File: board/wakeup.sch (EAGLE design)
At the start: 41 parts, among them IC2 ATMEGA48/88/168-AU, K1 PIN20X2, Q5 BC846BSMD, Q6 BC846BSMD, Q7 BC846BSMD, Q8 BC846BSMD, U1 EEPROM24

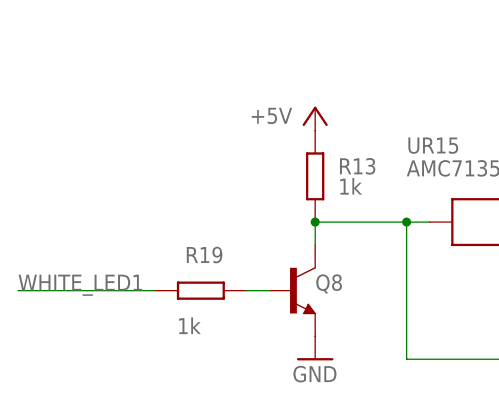
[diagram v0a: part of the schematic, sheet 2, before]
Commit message: Fixed some errors
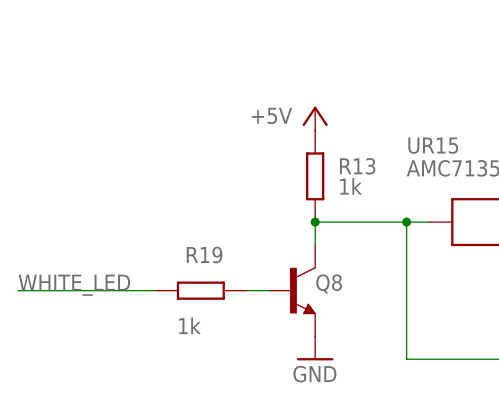
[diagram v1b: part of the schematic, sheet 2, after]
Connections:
- removed net WHITE_LED1: R19.2
- net WHITE_LED: now also R19.2
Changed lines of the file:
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@@
 <grid distance="0.1" unitdist="inch" unit="inch" style="lines" multiple="1" display="no" altdistance="0.01" altunitdist="inch" altunit="inch"/>
 <layers>
-<layer number="1" name="Top" color="4" fill="1" visible="yes" active="no"/>
-<layer number="2" name="Route2" color="1" fill="3" visible="yes" active="no"/>
-<layer number="3" name="Route3" color="4" fill="3" visible="yes" active="no"/>
-<layer number="4" name="Route4" color="1" fill="4" visible="yes" active="no"/>
-<layer number="5" name="Route5" color="4" fill="4" visible="yes" active="no"/>
-<layer number="6" name="Route6" color="1" fill="8" visible="yes" active="no"/>
-<layer number="7" name="Route7" color="4" fill="8" visible="yes" active="no"/>
-<layer number="8" name="Route8" color="1" fill="2" visible="yes" active="no"/>
-<layer number="9" name="Route9" color="4" fill="2" visible="yes" active="no"/>
-<layer number="10" name="Route10" color="1" fill="7" visible="yes" active="no"/>
-<layer number="11" name="Route11" color="4" fill="7" visible="yes" active="no"/>
-<layer number="12" name="Route12" color="1" fill="5" visible="yes" active="no"/>
-<layer number="13" name="Route13" color="4" fill="5" visible="yes" active="no"/>
-<layer number="14" name="Route14" color="1" fill="6" visible="yes" active="no"/>
-<layer number="15" name="Route15" color="4" fill="6" visible="yes" active="no"/>
-<layer number="16" name="Bottom" color="1" fill="1" visible="yes" active="no"/>
-<layer number="17" name="Pads" color="2" fill="1" visible="yes" active="no"/>
-<layer number="18" name="Vias" color="2" fill="1" visible="yes" active="no"/>
-<layer number="19" name="Unrouted" color="6" fill="1" visible="yes" active="no"/>
-<layer number="20" name="Dimension" color="15" fill="1" visible="yes" active="no"/>
-<layer number="21" name="tPlace" color="7" fill="1" visible="yes" active="no"/>
-<layer number="22" name="bPlace" color="7" fill="1" visible="yes" active="no"/>
-<layer number="23" name="tOrigins" color="15" fill="1" visible="yes" active="no"/>
-<layer number="24" name="bOrigins" color="15" fill="1" visible="yes" active="no"/>
-<layer number="25" name="tNames" color="7" fill="1" visible="yes" active="no"/>
-<layer number="26" name="bNames" color="7" fill="1" visible="yes" active="no"/>
-<layer number="27" name="tValues" color="7" fill="1" visible="yes" active="no"/>
-<layer number="28" name="bValues" color="7" fill="1" visible="yes" active="no"/>
+<layer number="1" name="Top" color="4" fill="1" visible="no" active="no"/>
+<layer number="2" name="Route2" color="1" fill="3" visible="no" active="no"/>
+<layer number="3" name="Route3" color="4" fill="3" visible="no" active="no"/>
+<layer number="4" name="Route4" color="1" fill="4" visible="no" active="no"/>
+<layer number="5" name="Route5" color="4" fill="4" visible="no" active="no"/>
+<layer number="6" name="Route6" color="1" fill="8" visible="no" active="no"/>
+<layer number="7" name="Route7" color="4" fill="8" visible="no" active="no"/>
+<layer number="8" name="Route8" color="1" fill="2" visible="no" active="no"/>
+<layer number="9" name="Route9" color="4" fill="2" visible="no" active="no"/>
+<layer number="10" name="Route10" color="1" fill="7" visible="no" active="no"/>
+<layer number="11" name="Route11" color="4" fill="7" visible="no" active="no"/>
+<layer number="12" name="Route12" color="1" fill="5" visible="no" active="no"/>
+<layer number="13" name="Route13" color="4" fill="5" visible="no" active="no"/>
+<layer number="14" name="Route14" color="1" fill="6" visible="no" active="no"/>
+<layer number="15" name="Route15" color="4" fill="6" visible="no" active="no"/>
+<layer number="16" name="Bottom" color="1" fill="1" visible="no" active="no"/>
+<layer number="17" name="Pads" color="2" fill="1" visible="no" active="no"/>
+<layer number="18" name="Vias" color="2" fill="1" visible="no" active="no"/>
+<layer number="19" name="Unrouted" color="6" fill="1" visible="no" active="no"/>
+<layer number="20" name="Dimension" color="15" fill="1" visible="no" active="no"/>
+<layer number="21" name="tPlace" color="7" fill="1" visible="no" active="no"/>
+<layer number="22" name="bPlace" color="7" fill="1" visible="no" active="no"/>
+<layer number="23" name="tOrigins" color="15" fill="1" visible="no" active="no"/>
+<layer number="24" name="bOrigins" color="15" fill="1" visible="no" active="no"/>
+<layer number="25" name="tNames" color="7" fill="1" visible="no" active="no"/>
+<layer number="26" name="bNames" color="7" fill="1" visible="no" active="no"/>
+<layer number="27" name="tValues" color="7" fill="1" visible="no" active="no"/>
+<layer number="28" name="bValues" color="7" fill="1" visible="no" active="no"/>
 <layer number="29" name="tStop" color="7" fill="3" visible="no" active="no"/>
 <layer number="30" name="bStop" color="7" fill="6" visible="no" active="no"/>
@@
 <layer number="35" name="tGlue" color="7" fill="4" visible="no" active="no"/>
 <layer number="36" name="bGlue" color="7" fill="5" visible="no" active="no"/>
-<layer number="37" name="tTest" color="7" fill="1" visible="yes" active="no"/>
-<layer number="38" name="bTest" color="7" fill="1" visible="yes" active="no"/>
+<layer number="37" name="tTest" color="7" fill="1" visible="no" active="no"/>
+<layer number="38" name="bTest" color="7" fill="1" visible="no" active="no"/>
 <layer number="39" name="tKeepout" color="4" fill="11" visible="no" active="no"/>
 <layer number="40" name="bKeepout" color="1" fill="11" visible="no" active="no"/>
@@
 <layer number="44" name="Drills" color="7" fill="1" visible="no" active="no"/>
 <layer number="45" name="Holes" color="7" fill="1" visible="no" active="no"/>
-<layer number="46" name="Milling" color="3" fill="1" visible="yes" active="no"/>
-<layer number="47" name="Measures" color="7" fill="1" visible="yes" active="no"/>
-<layer number="48" name="Document" color="7" fill="1" visible="yes" active="no"/>
-<layer number="49" name="Reference" color="7" fill="1" visible="yes" active="no"/>
-<layer number="50" name="dxf" color="7" fill="1" visible="yes" active="no"/>
-<layer number="51" name="tDocu" color="7" fill="1" visible="yes" active="no"/>
-<layer number="52" name="bDocu" color="7" fill="1" visible="yes" active="no"/>
-<layer number="53" name="tGND_GNDA" color="7" fill="1" visible="yes" active="no"/>
-<layer number="54" name="bGND_GNDA" color="7" fill="1" visible="yes" active="no"/>
-<layer number="56" name="wert" color="7" fill="1" visible="yes" active="no"/>
+<layer number="46" name="Milling" color="3" fill="1" visible="no" active="no"/>
+<layer number="47" name="Measures" color="7" fill="1" visible="no" active="no"/>
+<layer number="48" name="Document" color="7" fill="1" visible="no" active="no"/>
+<layer number="49" name="Reference" color="7" fill="1" visible="no" active="no"/>
+<layer number="50" name="dxf" color="7" fill="1" visible="no" active="no"/>
+<layer number="51" name="tDocu" color="7" fill="1" visible="no" active="no"/>
+<layer number="52" name="bDocu" color="7" fill="1" visible="no" active="no"/>
+<layer number="53" name="tGND_GNDA" color="7" fill="1" visible="no" active="no"/>
+<layer number="54" name="bGND_GNDA" color="7" fill="1" visible="no" active="no"/>
+<layer number="56" name="wert" color="7" fill="1" visible="no" active="no"/>
 <layer number="90" name="Modules" color="5" fill="1" visible="yes" active="yes"/>
 <layer number="91" name="Nets" color="2" fill="1" visible="yes" active="yes"/>
@@
 </segment>
 </net>
-<net name="WHITE_LED1" class="0">
+<net name="WHITE_LED" class="0">
 <segment>
 <wire x1="27.94" y1="38.1" x2="43.18" y2="38.1" width="0.1524" layer="91"/>

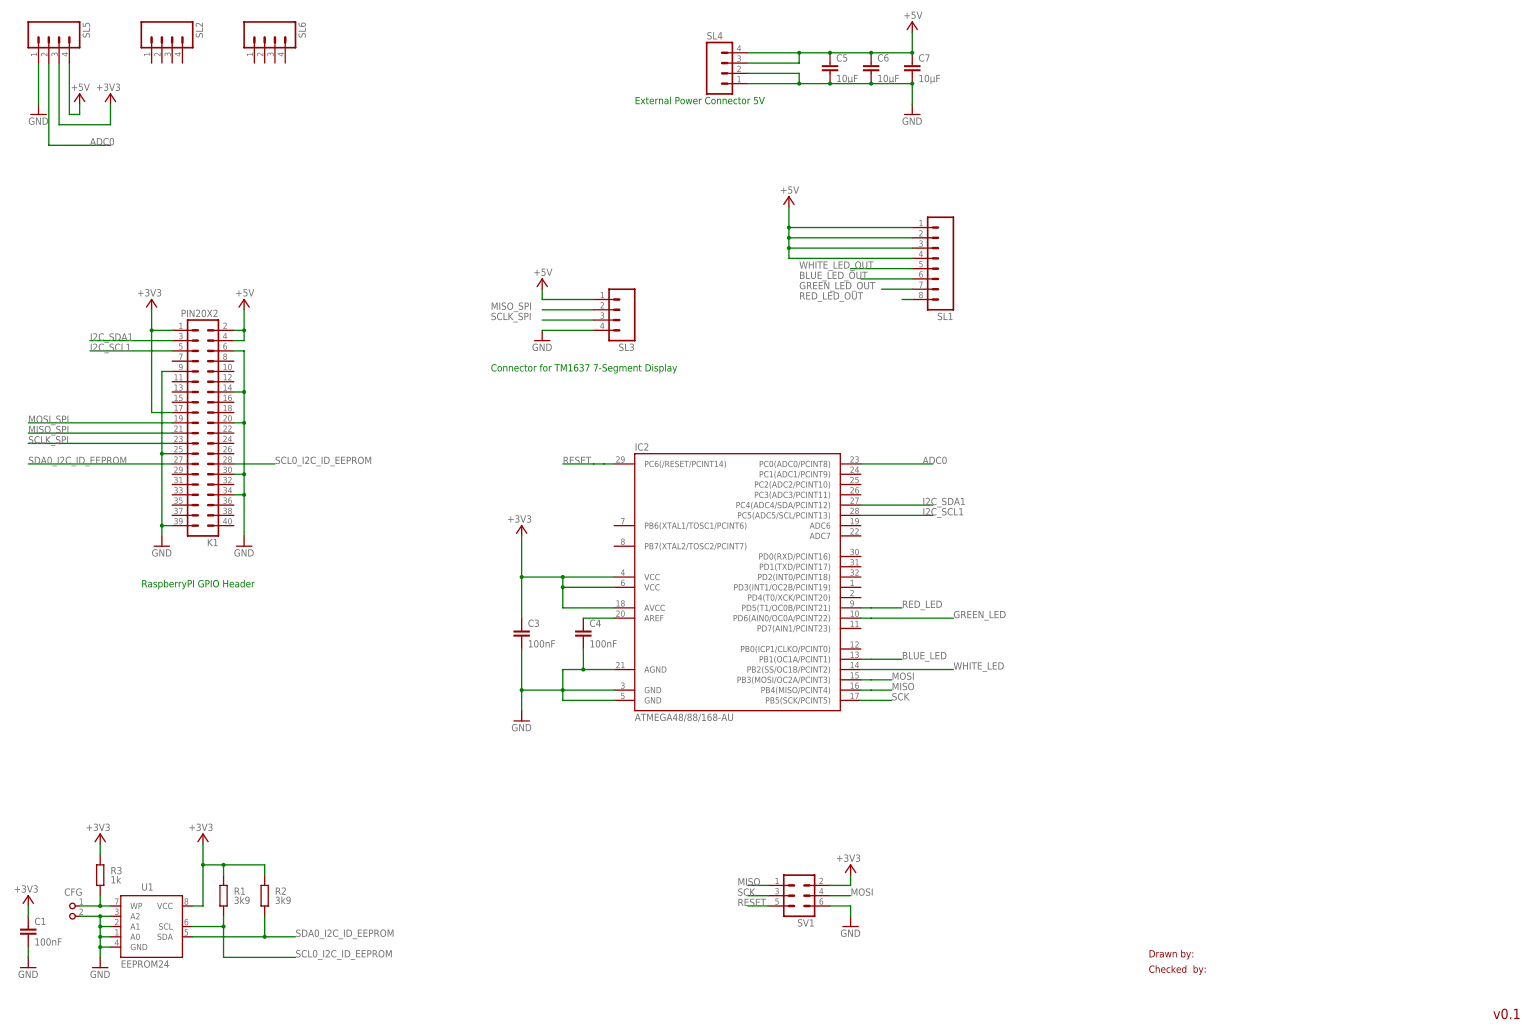
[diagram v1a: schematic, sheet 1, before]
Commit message: Finalized Updates
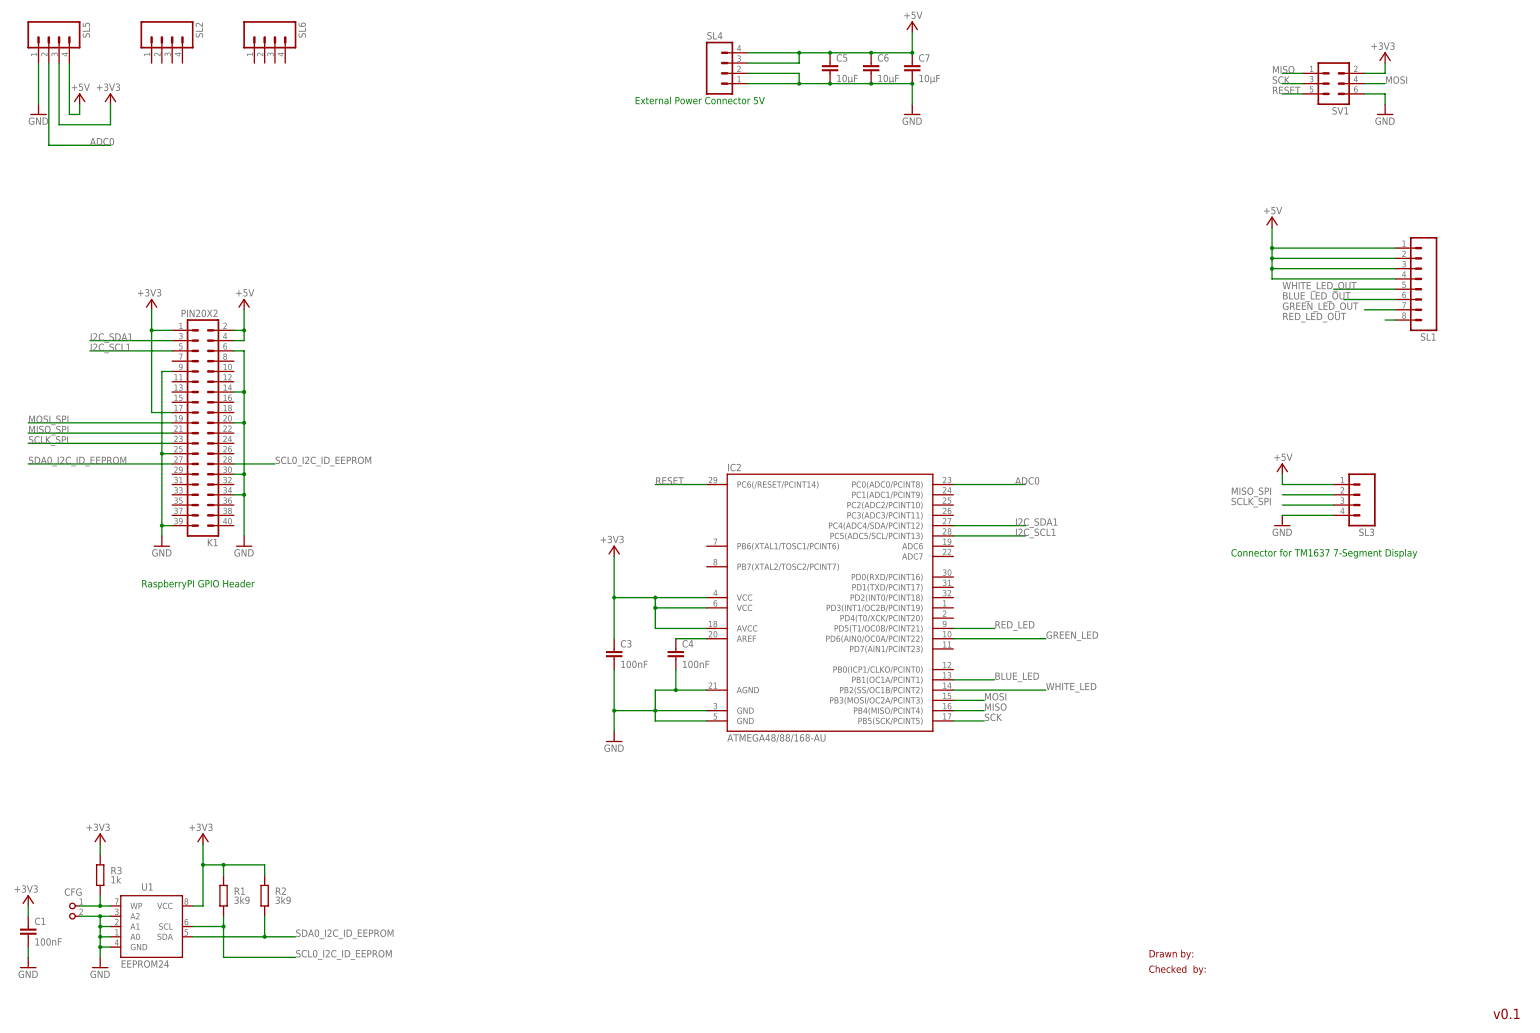
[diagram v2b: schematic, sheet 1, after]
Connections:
- net GLUMP1 renamed RED_POWER
- net SCHMARN1 renamed GREEN_POWER
- net TEST1 renamed BLUE_POWER
- net ZEUCH1 renamed WHITE_POWER
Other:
- moved on the sheet: C3, C4, IC2, SL1, SL3, SV1
